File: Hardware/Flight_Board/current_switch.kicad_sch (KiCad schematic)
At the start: 29 parts, among them U8 TPS274160A

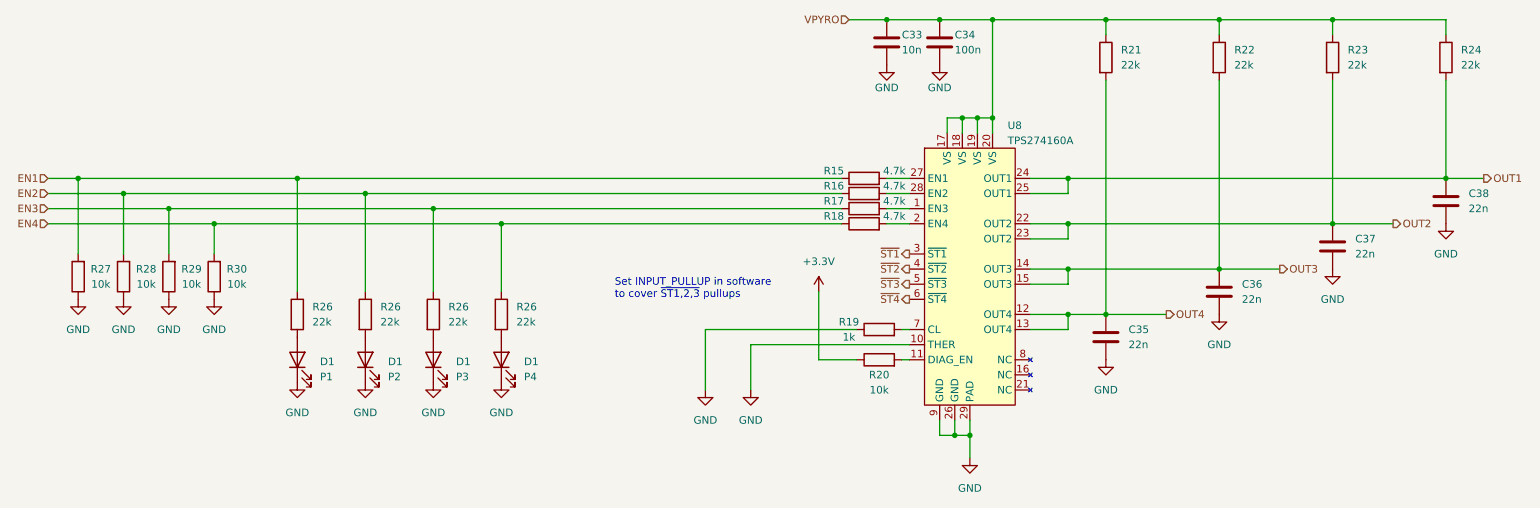
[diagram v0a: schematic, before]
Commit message: route buck and current switch
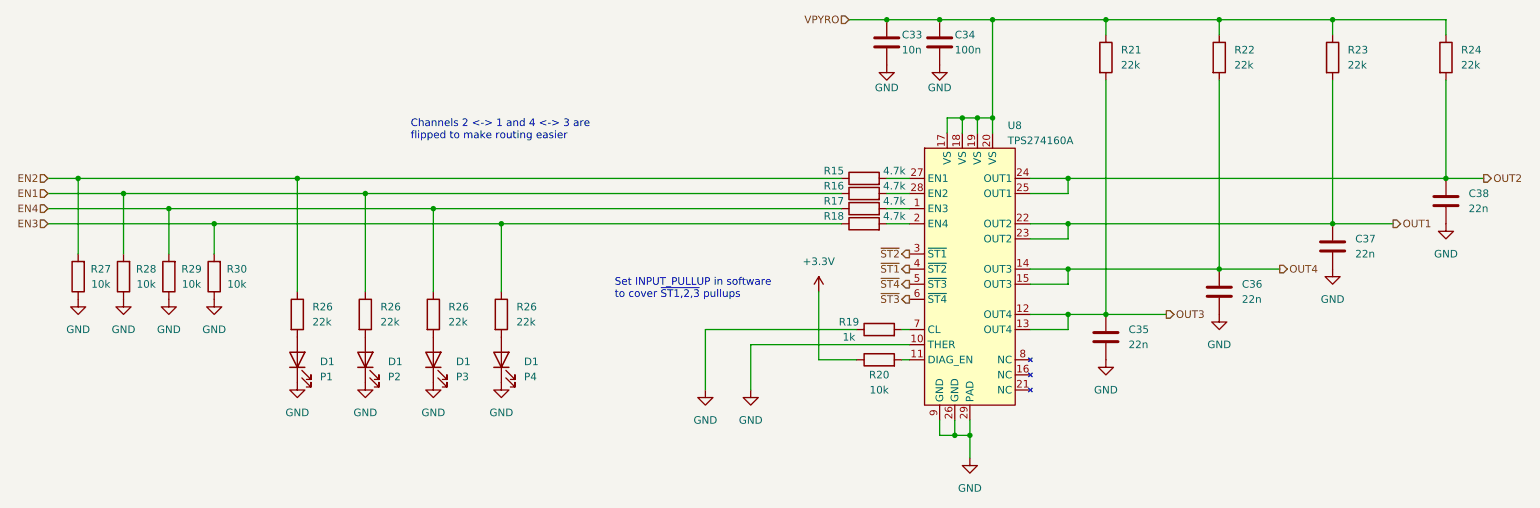
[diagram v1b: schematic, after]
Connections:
- net EN1: now also R16.1, R26.1, R28.2; no longer R15.1, R26.1, R27.2
- net EN2: now also R15.1, R26.1, R27.2; no longer R16.1, R26.1, R28.2
- net EN3: now also R18.1, R26.1, R30.2; no longer R17.1, R26.1, R29.2
- net EN4: now also R17.1, R26.1, R29.2; no longer R18.1, R26.1, R30.2
- net OUT1: now also C37.1, R23.2, U8.22 (OUT2), U8.23 (OUT2); no longer C38.1, R24.2, U8.24 (OUT1), U8.25 (OUT1)
- net OUT2: now also C38.1, R24.2, U8.24 (OUT1), U8.25 (OUT1); no longer C37.1, R23.2, U8.22 (OUT2), U8.23 (OUT2)
- net OUT3: now also C35.1, R21.2, U8.12 (OUT4), U8.13 (OUT4); no longer C36.1, R22.2, U8.14 (OUT3), U8.15 (OUT3)
- net OUT4: now also C36.1, R22.2, U8.14 (OUT3), U8.15 (OUT3); no longer C35.1, R21.2, U8.12 (OUT4), U8.13 (OUT4)
- net ~{ST1}: now also U8.4 (~{ST2}); no longer U8.3 (~{ST1})
- net ~{ST2}: now also U8.3 (~{ST1}); no longer U8.4 (~{ST2})
- net ~{ST3}: now also U8.6 (~{ST4}); no longer U8.5 (~{ST3})
- net ~{ST4}: now also U8.5 (~{ST3}); no longer U8.6 (~{ST4})
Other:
- note added: "Channels 2 <-> 1 and 4 <-> 3 are flipped to make routing easier"
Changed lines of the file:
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@@
     (stroke (width 0) (type default))
+  )
+  (text "Channels 2 <-> 1 and 4 <-> 3 are\nflipped to make routing easier"
+    (at 88.9 77.47 0)
+    (effects (font (size 1.27 1.27)) (justify left bottom))
   )
   (text "Set INPUT_PULLUP in software\nto cover ~{ST1,2,3} pullups\n"
@@
     (effects (font (size 1.27 1.27)) (justify left bottom))
   )
-  (hierarchical_label "EN2" (shape input) (at 27.94 86.36 180) (fields_autoplaced)
+  (hierarchical_label "EN2" (shape input) (at 27.94 83.82 180) (fields_autoplaced)
     (effects (font (size 1.27 1.27)) (justify right))
   )
-  (hierarchical_label "OUT1" (shape output) (at 269.24 83.82 0) (fields_autoplaced)
+  (hierarchical_label "OUT1" (shape output) (at 254 91.44 0) (fields_autoplaced)
     (effects (font (size 1.27 1.27)) (justify left))
   )
-  (hierarchical_label "EN4" (shape input) (at 27.94 91.44 180) (fields_autoplaced)
+  (hierarchical_label "EN4" (shape input) (at 27.94 88.9 180) (fields_autoplaced)
     (effects (font (size 1.27 1.27)) (justify right))
   )
-  (hierarchical_label "~{ST1}" (shape output) (at 172.72 96.52 180) (fields_autoplaced)
+  (hierarchical_label "~{ST1}" (shape output) (at 172.72 99.06 180) (fields_autoplaced)
     (effects (font (size 1.27 1.27)) (justify right))
   )
-  (hierarchical_label "OUT4" (shape output) (at 215.9 106.68 0) (fields_autoplaced)
+  (hierarchical_label "OUT4" (shape output) (at 234.95 99.06 0) (fields_autoplaced)
     (effects (font (size 1.27 1.27)) (justify left))
   )
-  (hierarchical_label "EN1" (shape input) (at 27.94 83.82 180) (fields_autoplaced)
+  (hierarchical_label "EN1" (shape input) (at 27.94 86.36 180) (fields_autoplaced)
     (effects (font (size 1.27 1.27)) (justify right))
   )
-  (hierarchical_label "~{ST2}" (shape output) (at 172.72 99.06 180) (fields_autoplaced)
+  (hierarchical_label "~{ST2}" (shape output) (at 172.72 96.52 180) (fields_autoplaced)
     (effects (font (size 1.27 1.27)) (justify right))
   )
-  (hierarchical_label "OUT3" (shape output) (at 234.95 99.06 0) (fields_autoplaced)
+  (hierarchical_label "OUT3" (shape output) (at 215.9 106.68 0) (fields_autoplaced)
     (effects (font (size 1.27 1.27)) (justify left))
   )
-  (hierarchical_label "OUT2" (shape output) (at 254 91.44 0) (fields_autoplaced)
+  (hierarchical_label "OUT2" (shape output) (at 269.24 83.82 0) (fields_autoplaced)
     (effects (font (size 1.27 1.27)) (justify left))
   )
-  (hierarchical_label "~{ST3}" (shape output) (at 172.72 101.6 180) (fields_autoplaced)
+  (hierarchical_label "~{ST3}" (shape output) (at 172.72 104.14 180) (fields_autoplaced)
     (effects (font (size 1.27 1.27)) (justify right))
   )
-  (hierarchical_label "~{ST4}" (shape output) (at 172.72 104.14 180) (fields_autoplaced)
+  (hierarchical_label "~{ST4}" (shape output) (at 172.72 101.6 180) (fields_autoplaced)
     (effects (font (size 1.27 1.27)) (justify right))
   )
-  (hierarchical_label "EN3" (shape input) (at 27.94 88.9 180) (fields_autoplaced)
+  (hierarchical_label "EN3" (shape input) (at 27.94 91.44 180) (fields_autoplaced)
     (effects (font (size 1.27 1.27)) (justify right))
   )

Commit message: initial placement on board, continue routing
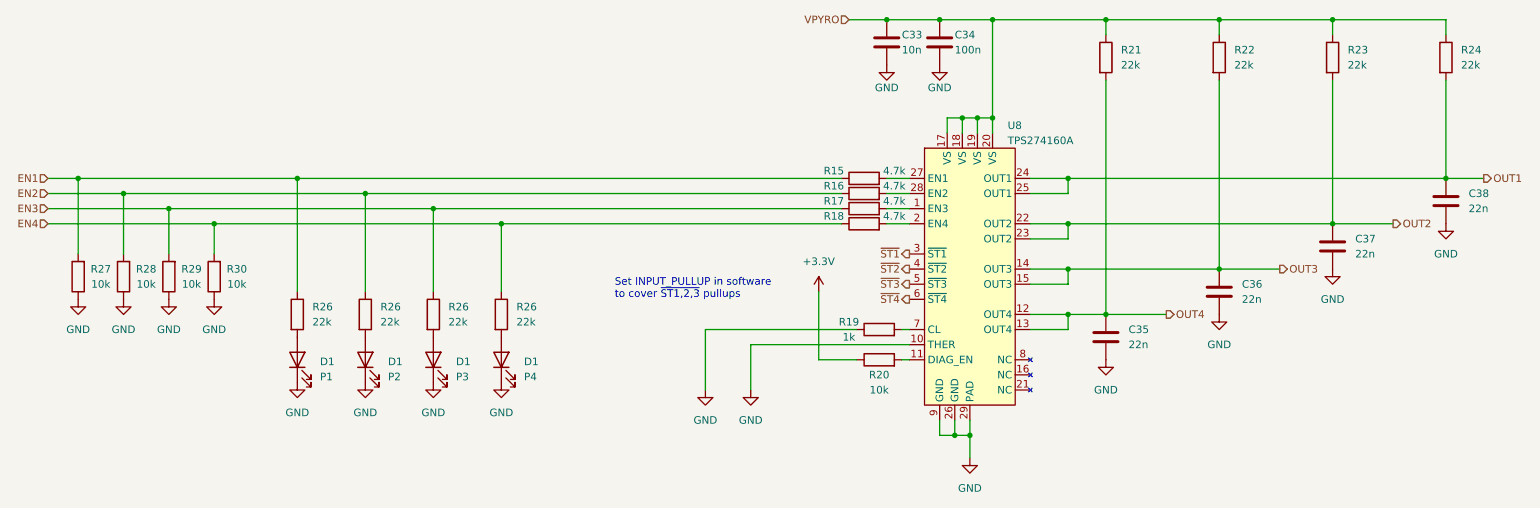
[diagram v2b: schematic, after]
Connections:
- net EN1: now also R15.1, R26.1, R27.2; no longer R16.1, R26.1, R28.2
- net EN2: now also R16.1, R26.1, R28.2; no longer R15.1, R26.1, R27.2
- net EN3: now also R17.1, R26.1, R29.2; no longer R18.1, R26.1, R30.2
- net EN4: now also R18.1, R26.1, R30.2; no longer R17.1, R26.1, R29.2
- net OUT1: now also C38.1, R24.2, U8.24 (OUT1), U8.25 (OUT1); no longer C37.1, R23.2, U8.22 (OUT2), U8.23 (OUT2)
- net OUT2: now also C37.1, R23.2, U8.22 (OUT2), U8.23 (OUT2); no longer C38.1, R24.2, U8.24 (OUT1), U8.25 (OUT1)
- net OUT3: now also C36.1, R22.2, U8.14 (OUT3), U8.15 (OUT3); no longer C35.1, R21.2, U8.12 (OUT4), U8.13 (OUT4)
- net OUT4: now also C35.1, R21.2, U8.12 (OUT4), U8.13 (OUT4); no longer C36.1, R22.2, U8.14 (OUT3), U8.15 (OUT3)
- net ~{ST1}: now also U8.3 (~{ST1}); no longer U8.4 (~{ST2})
- net ~{ST2}: now also U8.4 (~{ST2}); no longer U8.3 (~{ST1})
- net ~{ST3}: now also U8.5 (~{ST3}); no longer U8.6 (~{ST4})
- net ~{ST4}: now also U8.6 (~{ST4}); no longer U8.5 (~{ST3})
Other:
- note removed: "Channels 2 <-> 1 and 4 <-> 3 are flipped to make routing easier"
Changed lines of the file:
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@@
     (stroke (width 0) (type default))
-  )
-  (text "Channels 2 <-> 1 and 4 <-> 3 are\nflipped to make routing easier"
-    (at 88.9 77.47 0)
-    (effects (font (size 1.27 1.27)) (justify left bottom))
   )
   (text "Set INPUT_PULLUP in software\nto cover ~{ST1,2,3} pullups\n"
@@
     (effects (font (size 1.27 1.27)) (justify left bottom))
   )
-  (hierarchical_label "EN2" (shape input) (at 27.94 83.82 180) (fields_autoplaced)
+  (hierarchical_label "EN2" (shape input) (at 27.94 86.36 180) (fields_autoplaced)
     (effects (font (size 1.27 1.27)) (justify right))
   )
-  (hierarchical_label "OUT1" (shape output) (at 254 91.44 0) (fields_autoplaced)
+  (hierarchical_label "OUT1" (shape output) (at 269.24 83.82 0) (fields_autoplaced)
     (effects (font (size 1.27 1.27)) (justify left))
   )
-  (hierarchical_label "EN4" (shape input) (at 27.94 88.9 180) (fields_autoplaced)
+  (hierarchical_label "EN4" (shape input) (at 27.94 91.44 180) (fields_autoplaced)
     (effects (font (size 1.27 1.27)) (justify right))
   )
-  (hierarchical_label "~{ST1}" (shape output) (at 172.72 99.06 180) (fields_autoplaced)
+  (hierarchical_label "~{ST1}" (shape output) (at 172.72 96.52 180) (fields_autoplaced)
     (effects (font (size 1.27 1.27)) (justify right))
   )
-  (hierarchical_label "OUT4" (shape output) (at 234.95 99.06 0) (fields_autoplaced)
+  (hierarchical_label "OUT4" (shape output) (at 215.9 106.68 0) (fields_autoplaced)
     (effects (font (size 1.27 1.27)) (justify left))
   )
-  (hierarchical_label "EN1" (shape input) (at 27.94 86.36 180) (fields_autoplaced)
+  (hierarchical_label "EN1" (shape input) (at 27.94 83.82 180) (fields_autoplaced)
     (effects (font (size 1.27 1.27)) (justify right))
   )
-  (hierarchical_label "~{ST2}" (shape output) (at 172.72 96.52 180) (fields_autoplaced)
+  (hierarchical_label "~{ST2}" (shape output) (at 172.72 99.06 180) (fields_autoplaced)
     (effects (font (size 1.27 1.27)) (justify right))
   )
-  (hierarchical_label "OUT3" (shape output) (at 215.9 106.68 0) (fields_autoplaced)
+  (hierarchical_label "OUT3" (shape output) (at 234.95 99.06 0) (fields_autoplaced)
     (effects (font (size 1.27 1.27)) (justify left))
   )
-  (hierarchical_label "OUT2" (shape output) (at 269.24 83.82 0) (fields_autoplaced)
+  (hierarchical_label "OUT2" (shape output) (at 254 91.44 0) (fields_autoplaced)
     (effects (font (size 1.27 1.27)) (justify left))
   )
-  (hierarchical_label "~{ST3}" (shape output) (at 172.72 104.14 180) (fields_autoplaced)
+  (hierarchical_label "~{ST3}" (shape output) (at 172.72 101.6 180) (fields_autoplaced)
     (effects (font (size 1.27 1.27)) (justify right))
   )
-  (hierarchical_label "~{ST4}" (shape output) (at 172.72 101.6 180) (fields_autoplaced)
+  (hierarchical_label "~{ST4}" (shape output) (at 172.72 104.14 180) (fields_autoplaced)
     (effects (font (size 1.27 1.27)) (justify right))
   )
-  (hierarchical_label "EN3" (shape input) (at 27.94 91.44 180) (fields_autoplaced)
+  (hierarchical_label "EN3" (shape input) (at 27.94 88.9 180) (fields_autoplaced)
     (effects (font (size 1.27 1.27)) (justify right))
   )
